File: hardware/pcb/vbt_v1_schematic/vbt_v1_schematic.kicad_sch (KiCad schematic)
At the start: 10 parts, among them Q1 AO3401A, SW1 SW_SPST, SW2 SW_SPST

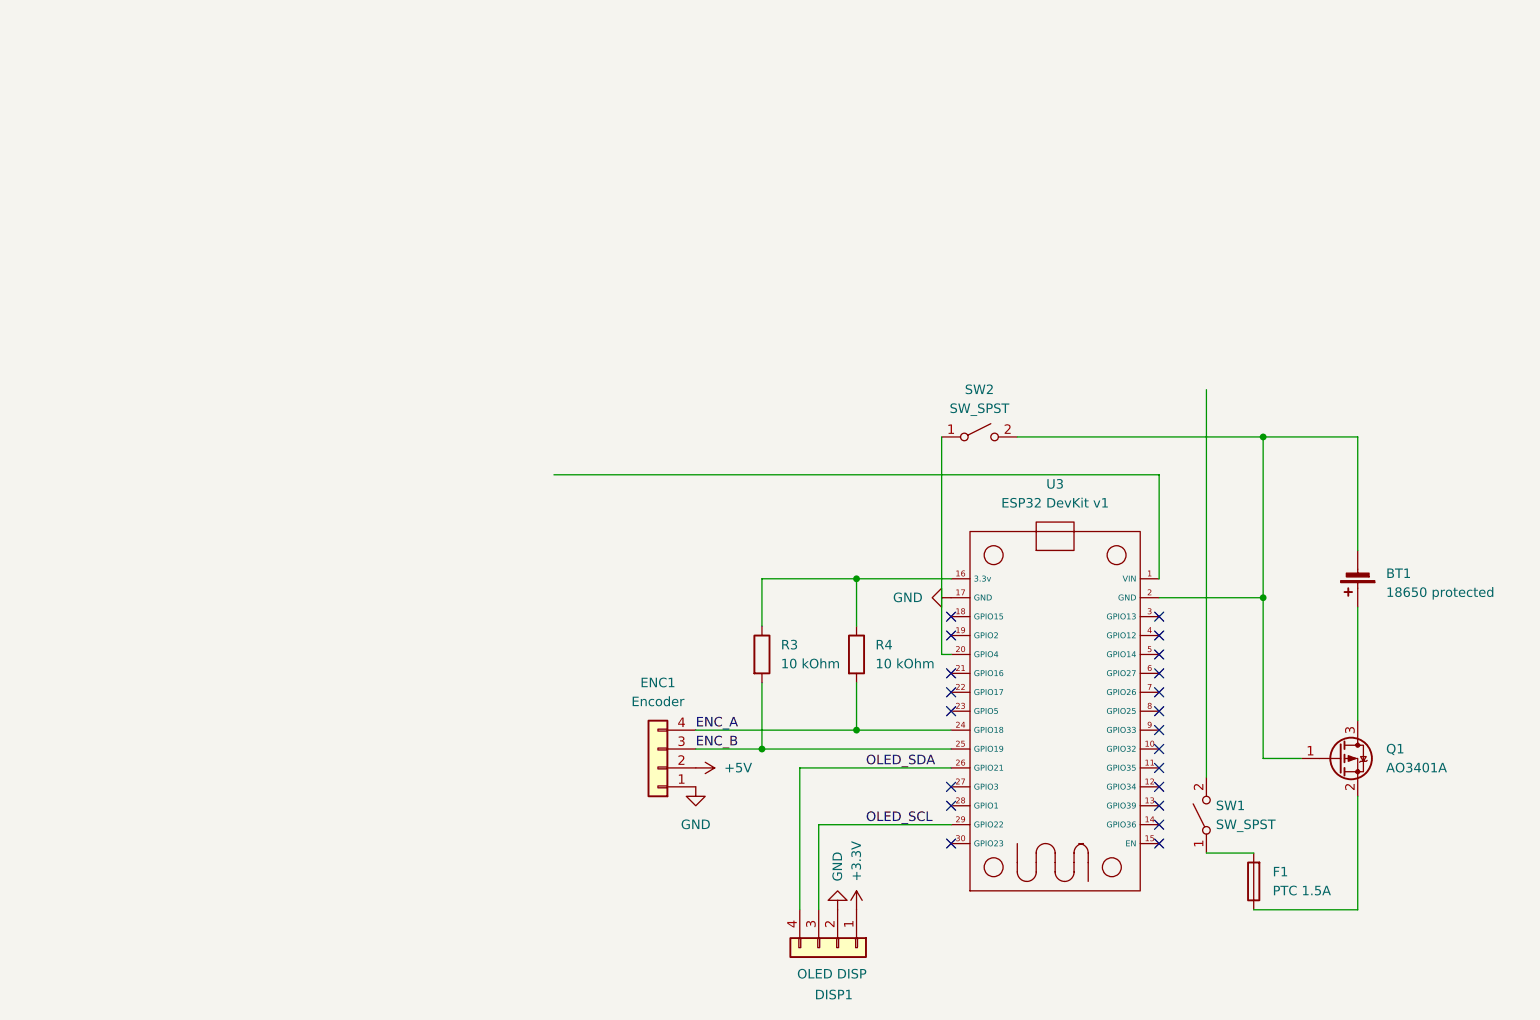
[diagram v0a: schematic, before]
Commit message: update: pcb layout complete
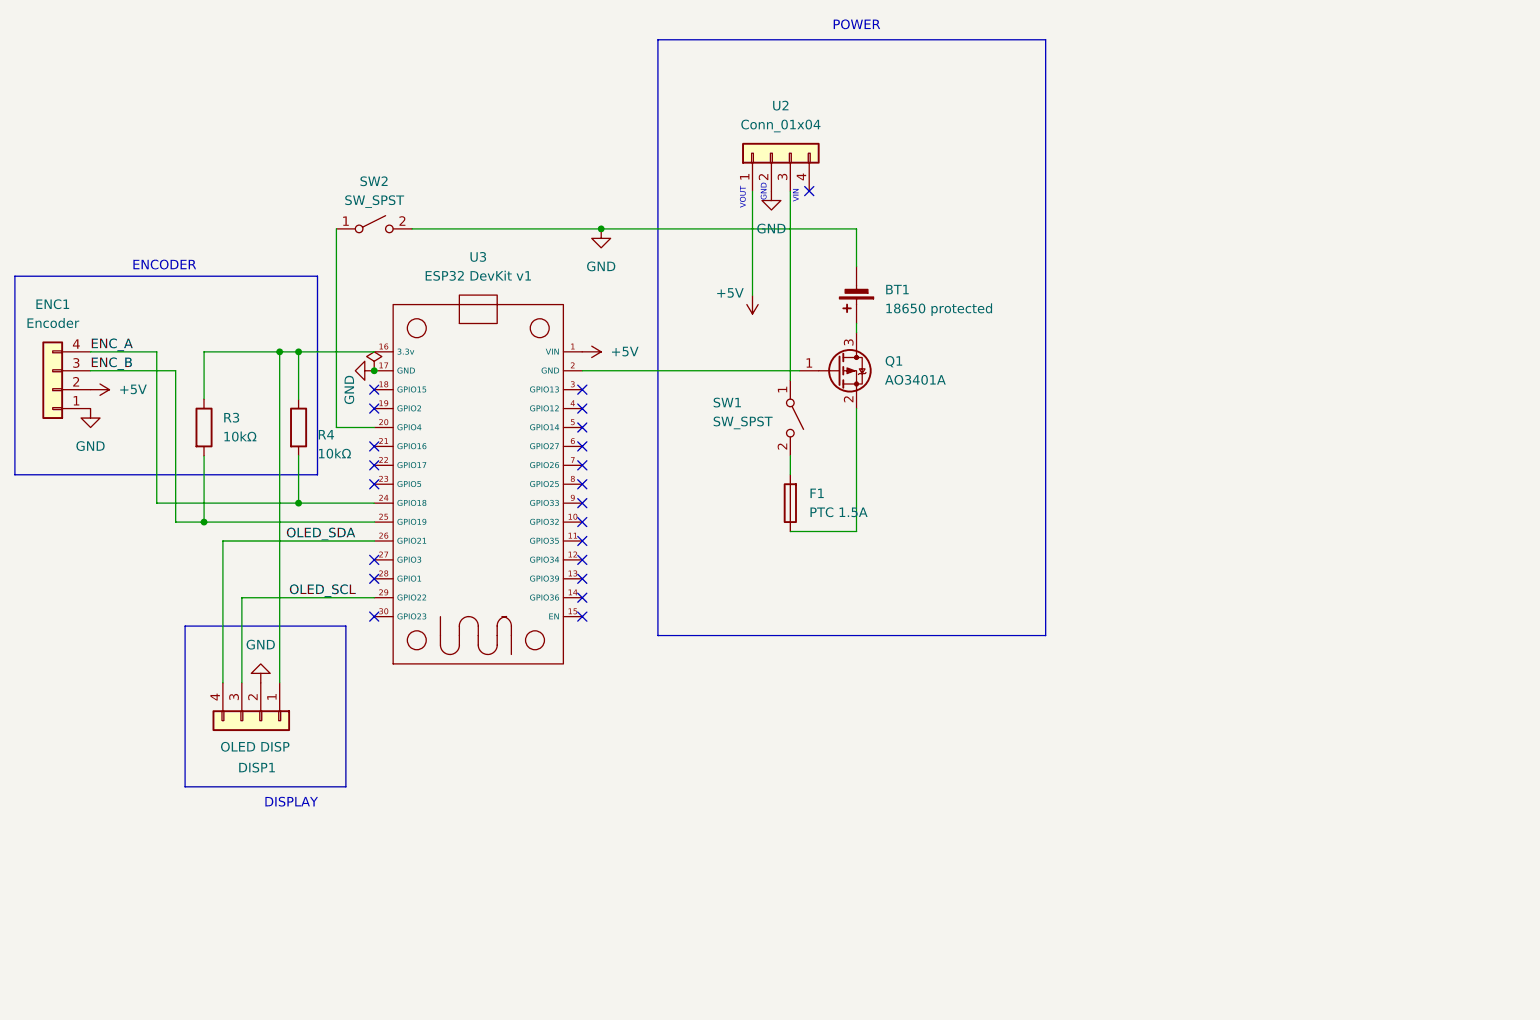
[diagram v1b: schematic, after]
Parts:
- added U2: Conn_01x04, Connector_PinHeader_2.54mm:PinHeader_1x04_P2.54mm_Vertical, symbol Connector_Generic:Conn_01x04
- DISP1: footprint (none) -> Connector_PinSocket_2.54mm:PinSocket_1x04_P2.54mm_Vertical
- ENC1: footprint (none) -> Connector_PinHeader_2.54mm:PinHeader_1x04_P2.54mm_Vertical
- F1: footprint (none) -> Fuse:Fuse_1812_4532Metric_Pad1.30x3.40mm_HandSolder
- R3, R4: value 10 kOhm -> 10kΩ; footprint (none) -> Resistor_THT:R_Axial_DIN0207_L6.3mm_D2.5mm_P10.16mm_Horizontal
- SW1: footprint (none) -> Connector_PinHeader_2.54mm:PinHeader_1x02_P2.54mm_Vertical
- SW2: footprint (none) -> Button_Switch_THT:SW_PUSH_6mm
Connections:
- net +3.3V is gone; now on an unnamed net: DISP1.1 (Pin_1)
- net +5V: now also U3.1 (VIN), U2.1 (Pin_1)
- net GND: now also BT1.2 (-), SW2.2 (B), U2.2 (Pin_2)
- net at SW1.1 (A): now also U2.3 (Pin_3); no longer F1.2
- net at SW1.2 (B): now also F1.2
- net at Q1.1 (G), U3.2 (GND): no longer BT1.2 (-), SW2.2 (B)
- no-connect marks 21 -> 22
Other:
- note added: "DISPLAY"
- note added: "ENCODER"
- note added: "GND"
- note added: "POWER"
- note added: "VIN"
- note added: "VOUT"
- title: (none) -> VBT WIRING V1
- moved on the sheet: BT1, DISP1, ENC1, F1, Q1, R3, R4, SW1, SW2, U3
